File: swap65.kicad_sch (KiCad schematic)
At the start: 34 parts, among them J1 USB_C_Receptacle_USB2.0, SW1 SW_Push, SW2 SW_Push, U1 RP2040, U2 USBLC6-2SC6, U3 XC6206PxxxMR, U4 W25Q128JVS, Y1 12MHz

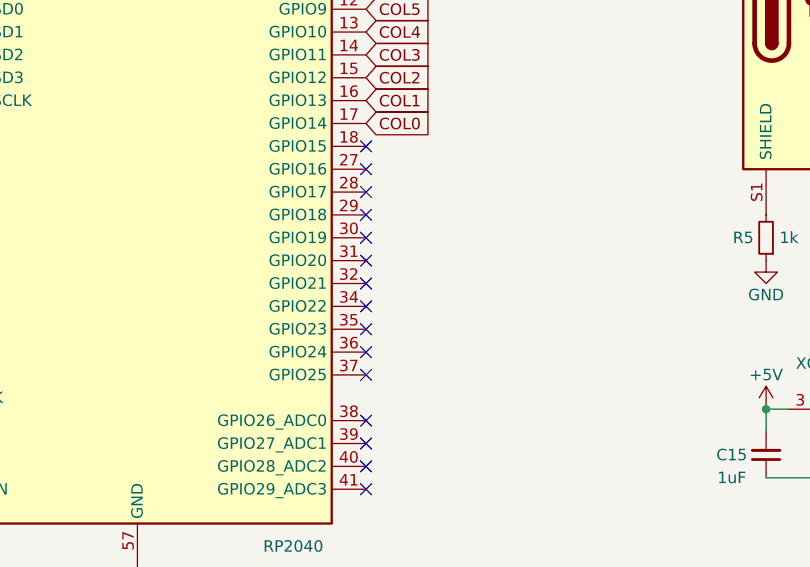
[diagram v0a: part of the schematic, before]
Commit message: completed first pass at routing
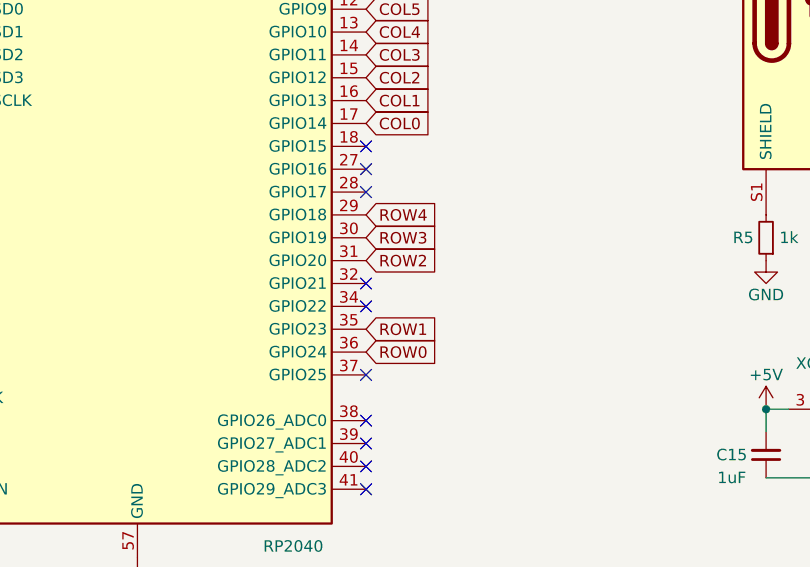
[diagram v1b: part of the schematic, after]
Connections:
- net ROW4: now reaches U1.29 (GPIO18)
- net ROW3: now reaches U1.30 (GPIO19)
- net ROW2: now reaches U1.31 (GPIO20)
- net ROW1: now reaches U1.35 (GPIO23)
- net ROW0: now reaches U1.36 (GPIO24)
- no-connect marks 19 -> 14
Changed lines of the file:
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@@
   (no_connect (at 100.33 113.03))
   (no_connect (at 100.33 120.65))
-  (no_connect (at 100.33 118.11))
   (no_connect (at 167.64 95.25))
   (no_connect (at 100.33 97.79))
   (no_connect (at 100.33 125.73))
-  (no_connect (at 100.33 105.41))
-  (no_connect (at 100.33 102.87))
   (no_connect (at 100.33 95.25))
   (no_connect (at 100.33 133.35))
@@
   (no_connect (at 100.33 128.27))
   (no_connect (at 49.53 125.73))
-  (no_connect (at 100.33 107.95))
-  (no_connect (at 100.33 115.57))
   (wire (pts (xy 165.1 124.46) (xy 165.1 127))
     (stroke (width 0) (type default) (color 0 0 0 0))
@@
     )
   )
+  (global_label "ROW3" (shape input) (at 100.33 105.41 0) (fields_autoplaced)
+    (effects (font (size 1.27 1.27)) (justify left))
+    (property "Intersheet References" "${INTERSHEET_REFS}" (id 0) (at 108.0045 105.3306 0)
+      (effects (font (size 1.27 1.27)) (justify left) hide)
+    )
+  )
   (global_label "QSPI_CLK" (shape input) (at 209.55 121.92 180) (fields_autoplaced)
     (effects (font (size 1.27 1.27)) (justify right))
@@
     )
   )
+  (global_label "ROW1" (shape input) (at 100.33 115.57 0) (fields_autoplaced)
+    (effects (font (size 1.27 1.27)) (justify left))
+    (property "Intersheet References" "${INTERSHEET_REFS}" (id 0) (at 108.0045 115.4906 0)
+      (effects (font (size 1.27 1.27)) (justify left) hide)
+    )
+  )
   (global_label "SD3" (shape input) (at 49.53 87.63 180) (fields_autoplaced)
     (effects (font (size 1.27 1.27)) (justify right))
@@
     )
   )
+  (global_label "ROW4" (shape input) (at 100.33 102.87 0) (fields_autoplaced)
+    (effects (font (size 1.27 1.27)) (justify left))
+    (property "Intersheet References" "${INTERSHEET_REFS}" (id 0) (at 108.0045 102.7906 0)
+      (effects (font (size 1.27 1.27)) (justify left) hide)
+    )
+  )
   (global_label "COL1" (shape input) (at 100.33 90.17 0) (fields_autoplaced)
     (effects (font (size 1.27 1.27)) (justify left))
@@
     )
   )
+  (global_label "ROW0" (shape input) (at 100.33 118.11 0) (fields_autoplaced)
+    (effects (font (size 1.27 1.27)) (justify left))
+    (property "Intersheet References" "${INTERSHEET_REFS}" (id 0) (at 108.0045 118.0306 0)
+      (effects (font (size 1.27 1.27)) (justify left) hide)
+    )
+  )
   (global_label "D_USB_P" (shape input) (at 170.18 83.82 0) (fields_autoplaced)
     (effects (font (size 1.27 1.27)) (justify left))
@@
       (effects (font (size 1.27 1.27)) (justify left) hide)
     )
+  )
+  (global_label "ROW2" (shape input) (at 100.33 107.95 0) (fields_autoplaced)
+    (effects (font (size 1.27 1.27)) (justify left))
+    (property "Intersheet References" "${INTERSHEET_REFS}" (id 0) (at 108.0045 107.8706 0)
+      (effects (font (size 1.27 1.27)) (justify left) hide)
+    )
